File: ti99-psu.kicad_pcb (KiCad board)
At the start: 2 copper layers, 8 parts, among them J1 DC +12V IN, J2 +12V OUT, J3 +12V OUT, J4 -5V Regulator Out, J5 +5V Regulator Out, J6 TI-99/4A Power

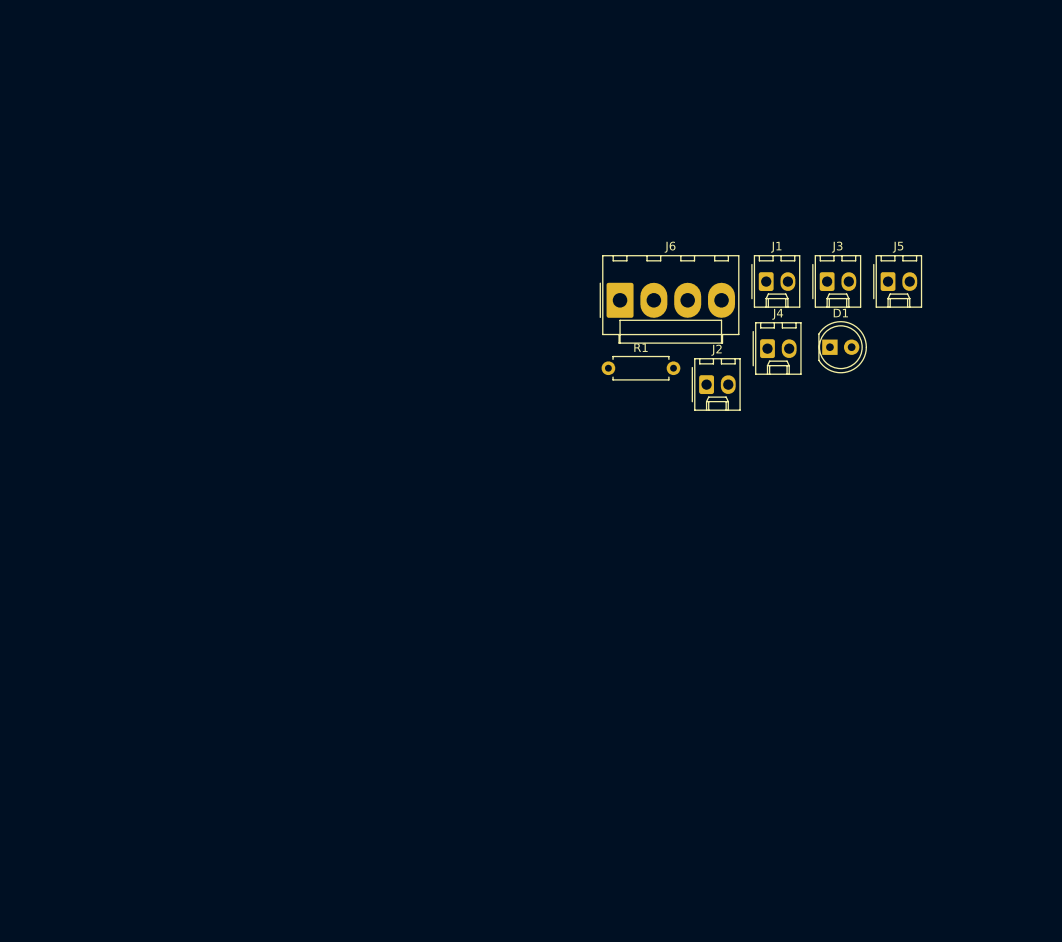
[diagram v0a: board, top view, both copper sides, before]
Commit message: V1 sent to production
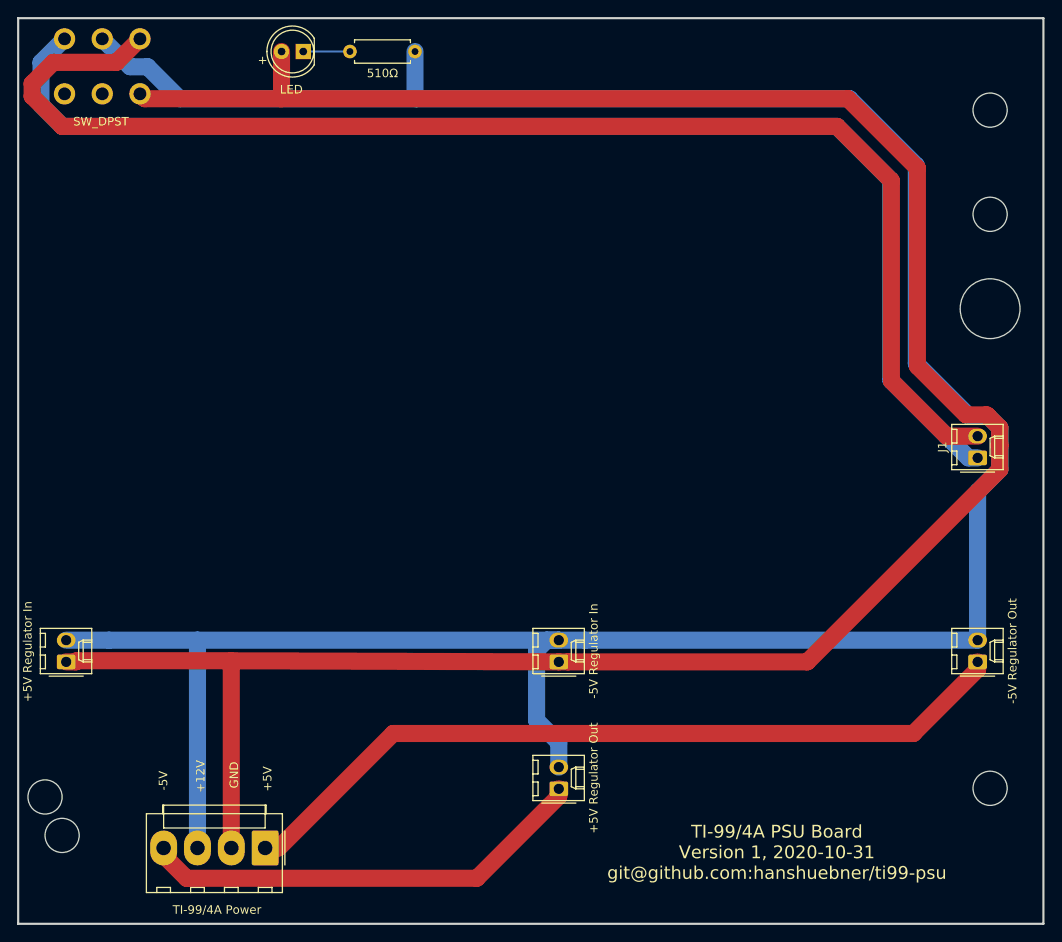
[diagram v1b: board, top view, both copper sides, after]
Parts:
- added ?: , AutoGenerated:MountingHole_4.00mm, F.Cu at (42.6, 143.4)
- added ?: , AutoGenerated:MountingHole_4.00mm, F.Cu at (40.6, 138.9)
- added ?: , AutoGenerated:MountingHole_4.00mm, F.Cu at (151.2, 70.7)
- added ?: , AutoGenerated:MountingHole_7.00mm, F.Cu at (151.2, 81.7)
- added ?: , AutoGenerated:MountingHole_4.00mm, F.Cu at (151.2, 137.9)
- added ?: , AutoGenerated:MountingHole_4.00mm, F.Cu at (151.2, 58.5)
- added SW1: SW_DPST, Button_Switch_THT:SW_Slider_DPST, F.Cu at (47.3, 45.5)
- J2: value +12V OUT -> -5V Regulator In
- J3: value +12V OUT -> +5V Regulator In
- moved J3 99.6 mm to (43.1, 123.1), turned to 90 degrees
- moved J6 76.4 mm to (66.3, 144.8), turned to 180 degrees
- moved J5 70.8 mm to (100.7, 137.9), turned to 90 degrees
- moved D1 70.7 mm to (70.8, 51.6), turned to 180 degrees
- moved R1 47.8 mm to (76.3, 51.6)
- moved J4 44.1 mm to (149.7, 123.1), turned to 90 degrees
- moved J2 36.8 mm to (100.7, 123.1), turned to 90 degrees
- moved J1 32.2 mm to (149.7, 99.2), turned to 90 degrees
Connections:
- J4 pad 2: Net-(J4-Pad2) -> GND
- J5 pad 2: Net-(J4-Pad2) -> GND
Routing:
- net GND: track 0.00 -> 317.9 mm
- net +12V: track 0.00 -> 281.8 mm
- net Net-(J1-Pad2): track 0.00 -> 157.2 mm
- net Net-(J1-Pad1): track 0.00 -> 149.3 mm
- net /-5V: track 0.00 -> 92.9 mm
- net /+5V: track 0.00 -> 53.1 mm
- net Net-(D1-Pad1): track 0.00 -> 5.46 mm
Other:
- board outline added: 120 x 106 mm
- net class 12V added: clearance 0.4, trace_width 0.75, via_dia 0.8, via_drill 0.4
- net class Power added: clearance 0.5, trace_width 1, via_dia 0.8, via_drill 0.4
- board text added: "+"
- board text added: "+12V"
- board text added: "+5V"
- board text added: "-5V"
- board text added: "GND"
- board text added: "TI-99/4A PSU Board Version 1, 2020-10-31 git@github.com:hanshuebner/ti99-psu"
